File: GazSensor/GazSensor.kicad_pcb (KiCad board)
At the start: 2 copper layers, 128.3 x 53.3 mm, 20 parts, among them P1 Power, P2 Analog, P3 Digital, P4 Digital, P5 CONN_01X01, P6 CONN_01X01, P7 CONN_01X01, P8 CONN_01X01, U101 RN2483_breakout, U102 LTC1050

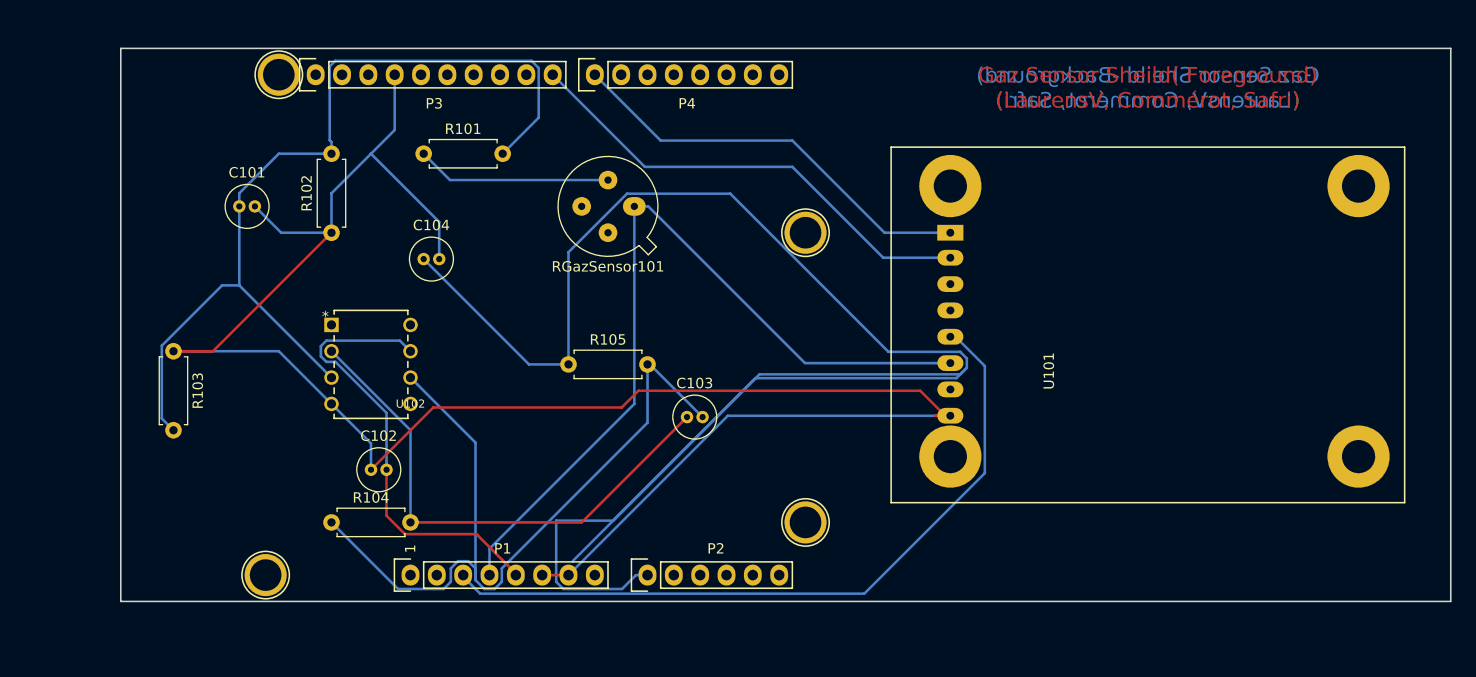
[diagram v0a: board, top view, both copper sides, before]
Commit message: New sheild
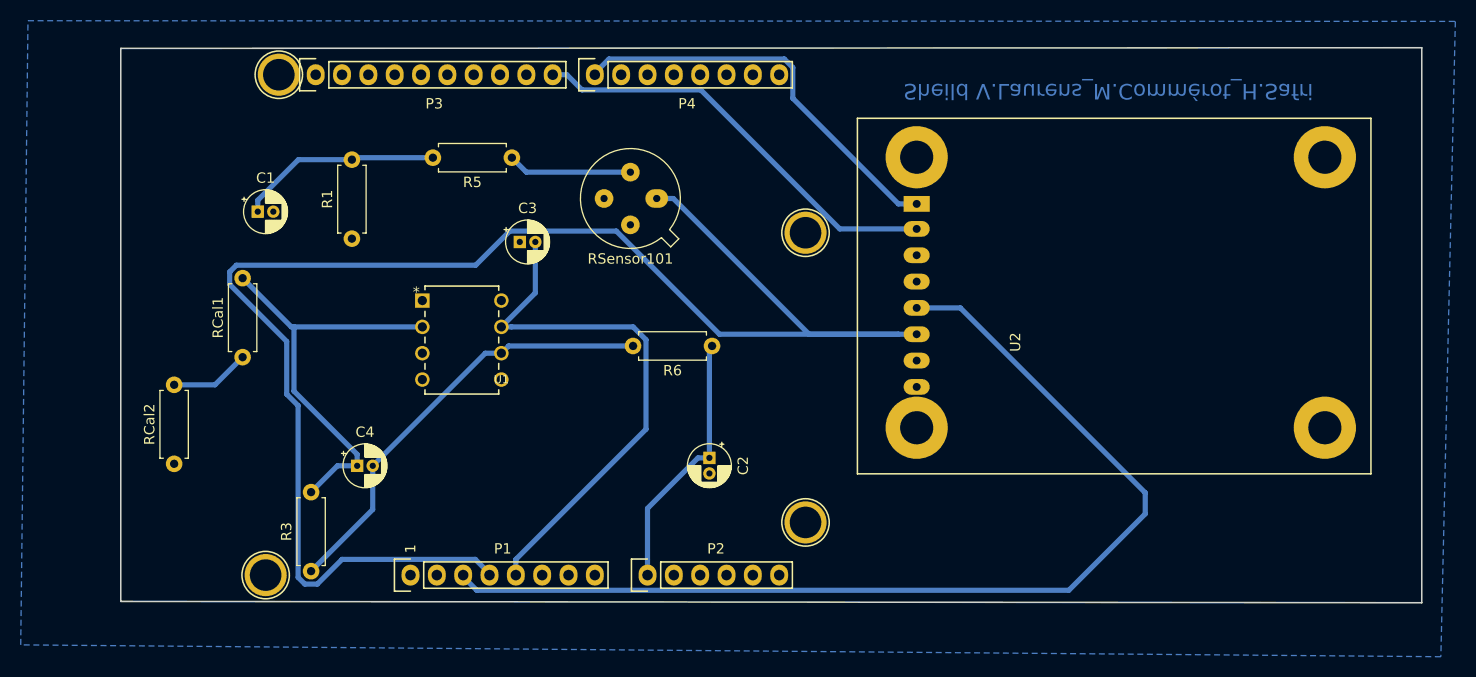
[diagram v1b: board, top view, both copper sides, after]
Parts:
- removed C101, C103, C104: 100n, Capacitor_THT:C_Radial_D4.0mm_H5.0mm_P1.50mm
- removed C102: 1u, Capacitor_THT:C_Radial_D4.0mm_H5.0mm_P1.50mm
- removed R101: 10k, Resistor_THT:R_Axial_DIN0207_L6.3mm_D2.5mm_P7.62mm_Horizontal
- removed R102, R104: 100k, Resistor_THT:R_Axial_DIN0207_L6.3mm_D2.5mm_P7.62mm_Horizontal
- removed R103, R105: 1k, Resistor_THT:R_Axial_DIN0207_L6.3mm_D2.5mm_P7.62mm_Horizontal
- removed RGazSensor101: R, MyComponents:GazSensor
- removed U101: RN2483_breakout, MyComponents:RN2483_Breakout
- removed U102: LTC1050, MyComponents:PDIP-8_N
- added C1: 100n, Capacitor_THT:CP_Radial_D4.0mm_P1.50mm, F.Cu at (124.2, 88.8)
- added C2: 100n, Capacitor_THT:CP_Radial_D4.0mm_P1.50mm, F.Cu at (167.8, 112.5)
- added C3: 1u, Capacitor_THT:CP_Radial_D4.0mm_P1.50mm, F.Cu at (149.5, 91.7)
- added C4: 1u, Capacitor_THT:CP_Radial_D4.0mm_P1.50mm, F.Cu at (133.8, 113.3)
- added R1: 100k, Resistor_THT:R_Axial_DIN0207_L6.3mm_D2.5mm_P7.62mm_Horizontal, F.Cu at (133.3, 91.4)
- added R3: 100k, Resistor_THT:R_Axial_DIN0207_L6.3mm_D2.5mm_P7.62mm_Horizontal, F.Cu at (129.3, 123.4)
- added R5: 10k, Resistor_THT:R_Axial_DIN0207_L6.3mm_D2.5mm_P7.62mm_Horizontal, F.Cu at (148.7, 83.6)
- added R6: 1k, Resistor_THT:R_Axial_DIN0207_L6.3mm_D2.5mm_P7.62mm_Horizontal, F.Cu at (168.0, 101.7)
- added RCal1: R, Resistor_THT:R_Axial_DIN0207_L6.3mm_D2.5mm_P7.62mm_Horizontal, F.Cu at (122.7, 102.8)
- added RCal2: R, Resistor_THT:R_Axial_DIN0207_L6.3mm_D2.5mm_P7.62mm_Horizontal, F.Cu at (116.1, 113.1)
- added RSensor101: R, MyComponents:GazSensor, F.Cu at (162.7, 87.5)
- added U1: LTC1050, MyComponents:PDIP-8_N, F.Cu at (147.7, 105.0)
- added U2: RN2483_breakout, MyComponents:RN2483_Breakout, F.Cu at (187.8, 88.0)
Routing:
- net GND: track 191.8 -> 0.00 mm
- net /A0: track 184.2 -> 25.3 mm
- net Net-(C101-Pad1): track 89.3 -> 0.00 mm
- net Net-(C103-Pad2): track 79.3 -> 0.00 mm
- net +3V3: track 78.1 -> 154.0 mm
- net Net-(C103-Pad1): track 50.5 -> 0.00 mm
- net Net-(C4-Pad2): track 0.00 -> 42.5 mm
- net Net-(C4-Pad1): track 0.00 -> 40.7 mm
- net /Reset: track 70.8 -> 101.5 mm
- net Net-(C1-Pad1): track 0.00 -> 19.7 mm
- net Net-(R101-Pad1): track 18.8 -> 0.00 mm
- net Net-(R5-Pad1): track 0.00 -> 12.0 mm
- net +5V: track 43.7 -> 51.9 mm
- net Net-(RCal1-Pad1): track 0.00 -> 7.71 mm
- net /8: track 45.7 -> 41.3 mm
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- added copper zone on B.Cu, net GND
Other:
- board size 128.3 x 53.3 mm -> 125.5 x 53.5 mm
- rule trace_min: 0.1 -> 0.2
- board text added: "Sheild V.Laurens_M.Commérot_H.Safri"
- board text removed: "Gaz Sensor Sheild -Background) (LaurensV, Commérot, Safri)"
- board text removed: "Gaz Sensor Sheild( Foreground) (LaurensV, Commérot, Safri)"
